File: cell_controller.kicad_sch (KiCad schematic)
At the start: 20 parts, among them Q1 BSS84, Q2 BSS84, U1 BQ78350DBT

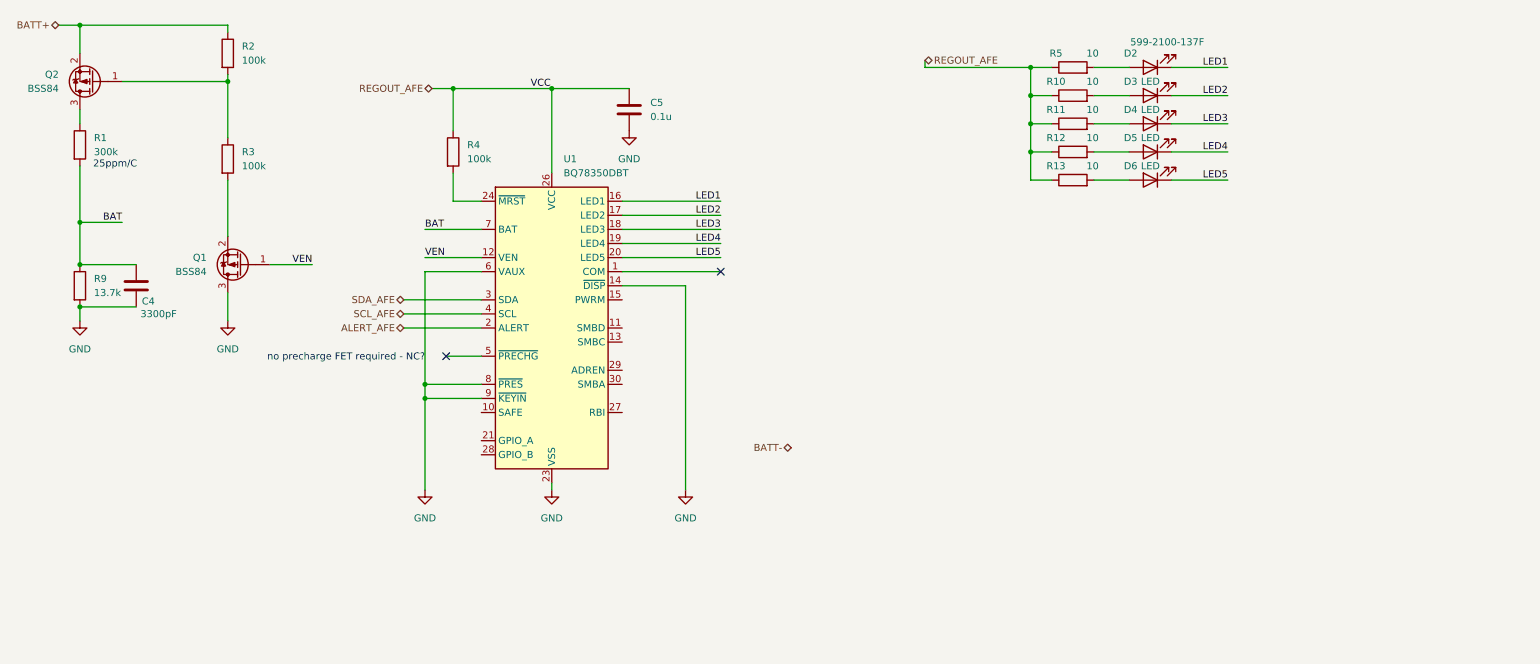
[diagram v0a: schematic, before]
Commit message: updates
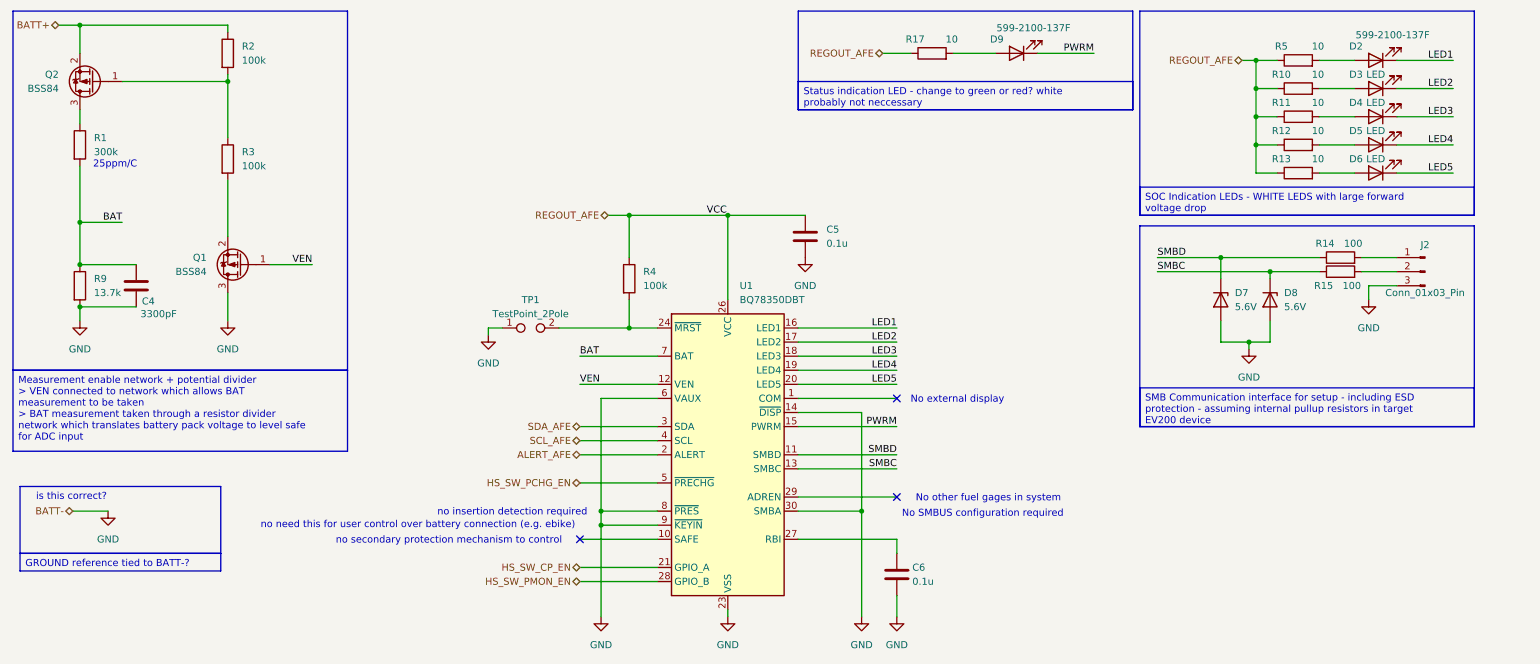
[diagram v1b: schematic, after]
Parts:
- added C6: 0.1u, symbol Device:C
- added D7, D8: 5.6V, symbol Device:D_Zener
- added D9: 599-2100-137F, LED_SMD:LED_1210_3225Metric, symbol Device:LED
- added J2: Conn_01x03_Pin, symbol Connector:Conn_01x03_Pin
- added R14, R15: 100, symbol Device:R
- added R17: 10, symbol Device:R
- added TP1: TestPoint_2Pole, Jumper:SolderJumper-2_P1.3mm_Open_RoundedPad1.0x1.5mm, symbol Connector:TestPoint_2Pole
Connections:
- net GND: now also U1.30 (SMBA), C6.2, D7.2 (A), D8.2 (A), J2.3 (Pin_3), TP1.1
- net REGOUT_AFE: now also R17.1
- net at R4.2, U1.24 (~{MRST}): now also TP1.2
- net SMBD: now reaches U1.11 (SMBD)
- net SMBD: now also D7.1 (K), R14.1
- net SMBC: now reaches U1.13 (SMBC)
- net SMBC: now also D8.1 (K), R15.1
- net PWRM: now reaches U1.15 (PWRM)
- net PWRM: now also D9.1 (K)
- net HS_SW_CP_EN: now reaches U1.21 (GPIO_A)
- net at U1.27 (RBI): now also C6.1
- net HS_SW_PMON_EN: now reaches U1.28 (GPIO_B)
- net HS_SW_PCHG_EN: now reaches U1.5 (~{PRECHG})
- new net: J2.2 (Pin_2), R15.2
- new net: D9.2 (A), R17.2
- new net: J2.1 (Pin_1), R14.2
- no-connect marks 2 -> 3
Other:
- note added: "No SMBUS configuration required"
- note added: "No external display"
- note added: "No other fuel gages in system"
- note added: "is this correct?"
- note added: "no insertion detection required"
- note added: "no need this for user control over battery connection (e.g. ebike)"
- note added: "no secondary protection mechanism to control"
- note removed: "no precharge FET required - NC?"
- moved on the sheet: C5, D2, D3, D4, D5, D6, R10, R11, R12, R13, R4, R5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
